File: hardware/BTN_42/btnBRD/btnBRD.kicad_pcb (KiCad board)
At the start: 2 copper layers, 113 parts, among them J1 Jack-DC, J10 Display Jumper, J2 MIDI-IN, J3 MIDI-OUT, J4 AudioJack2, J5 AudioJack2, J6 AudioJack2, J7 AudioJack2, J8 AudioJack2, J9 AudioJack2, SW1 SW_Push, SW10 SW_Push, SW11 SW_Push, SW12 SW_Push, SW13 SW_Push, SW14 SW_Push, SW15 SW_Push, SW16 SW_Push, SW17 SW_Push, SW18 SW_Push, SW19 SW_Push, SW2 SW_Push, SW20 SW_Push, SW21 SW_Push, SW22 SW_Push, SW23 SW_Push, SW24 SW_Push, SW25 SW_Push, SW26 SW_Push, SW27 SW_Push, SW28 SW_Push, SW29 SW_Push, SW3 SW_Push, SW30 SW_Push, SW31 SW_Push, SW32 SW_Push, SW33 SW_Push, SW34 SW_Push, SW35 SW_Push, SW36 SW_Push, SW37 SW_Push, SW38 SW_Push, SW39 SW_Push, SW4 SW_Push, SW40 SW_Push, SW41 SW_Push, SW42 SW_Push, SW43 SW_Push, SW44 SW_Push, SW45 SW_Push, SW46 SW_Push, SW47 SW_Push, SW48 SW_Push, SW5 SW_Push, SW6 SW_Push, SW7 SW_Push, SW8 SW_Push, SW9 SW_Push, U1 brain, U2 CD74HC4067M, U3 CD74HC4067M, U4 TXB0108DQSR

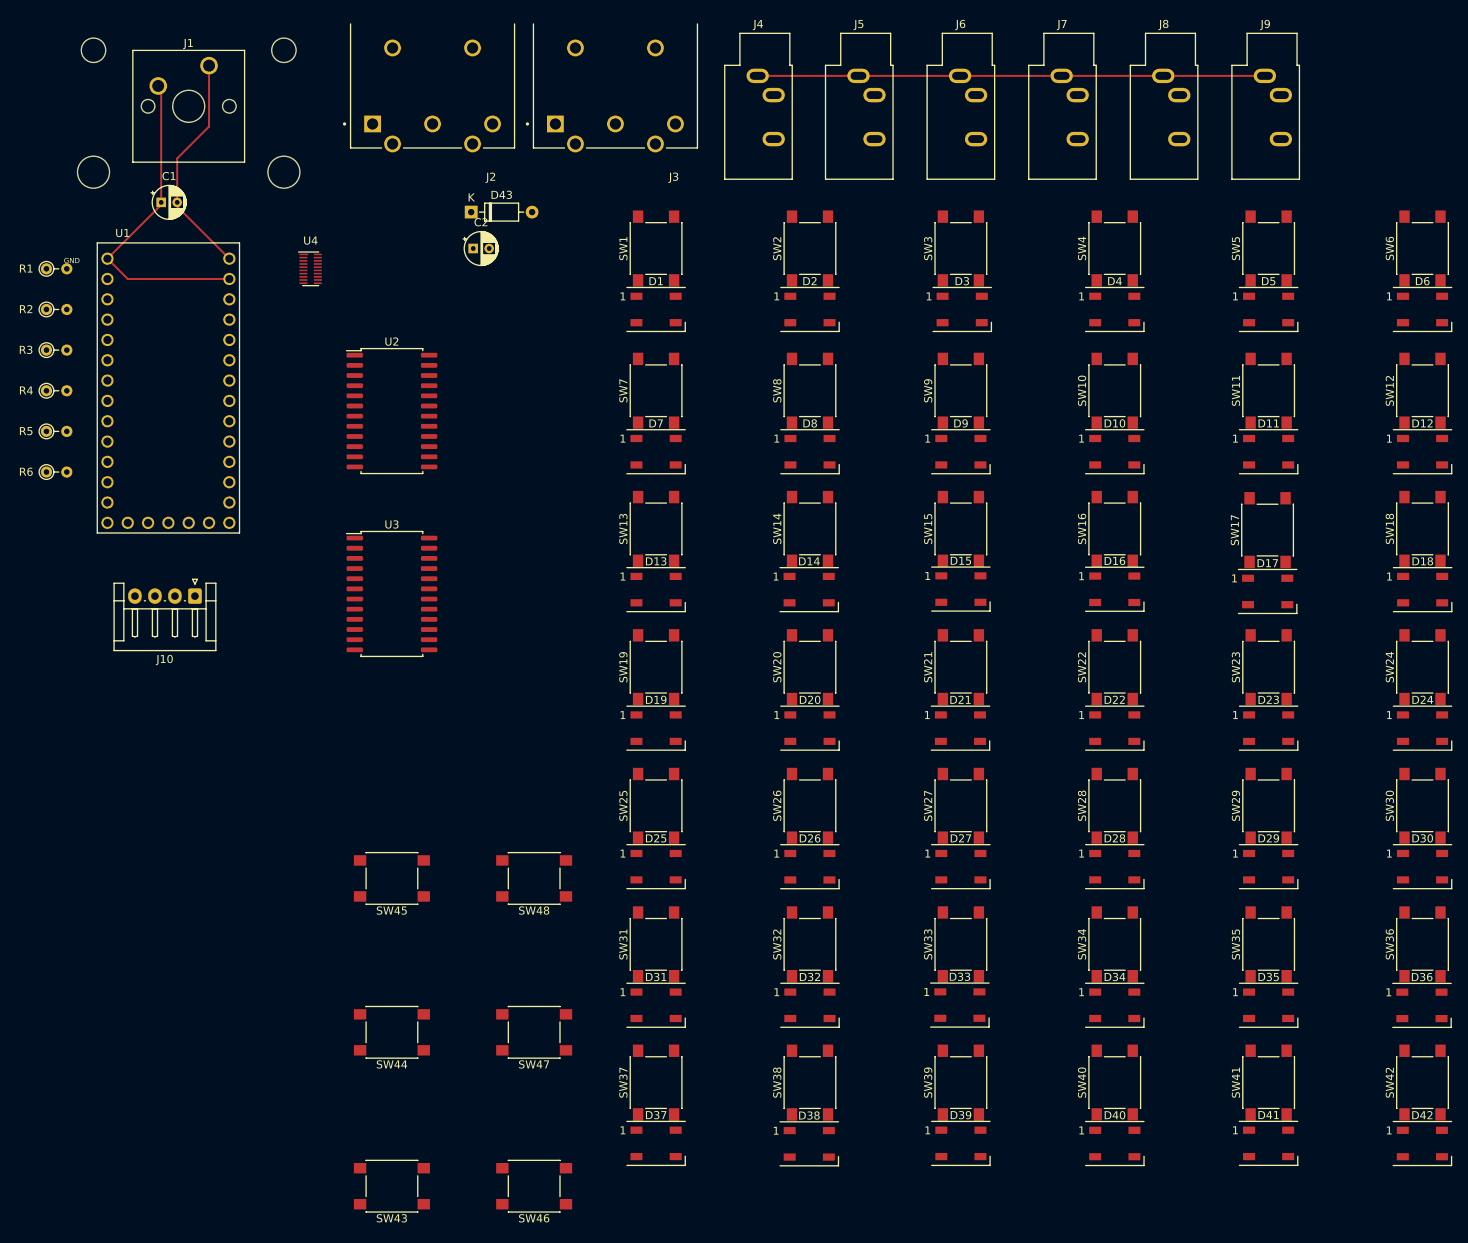
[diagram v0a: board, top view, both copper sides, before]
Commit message: brddd
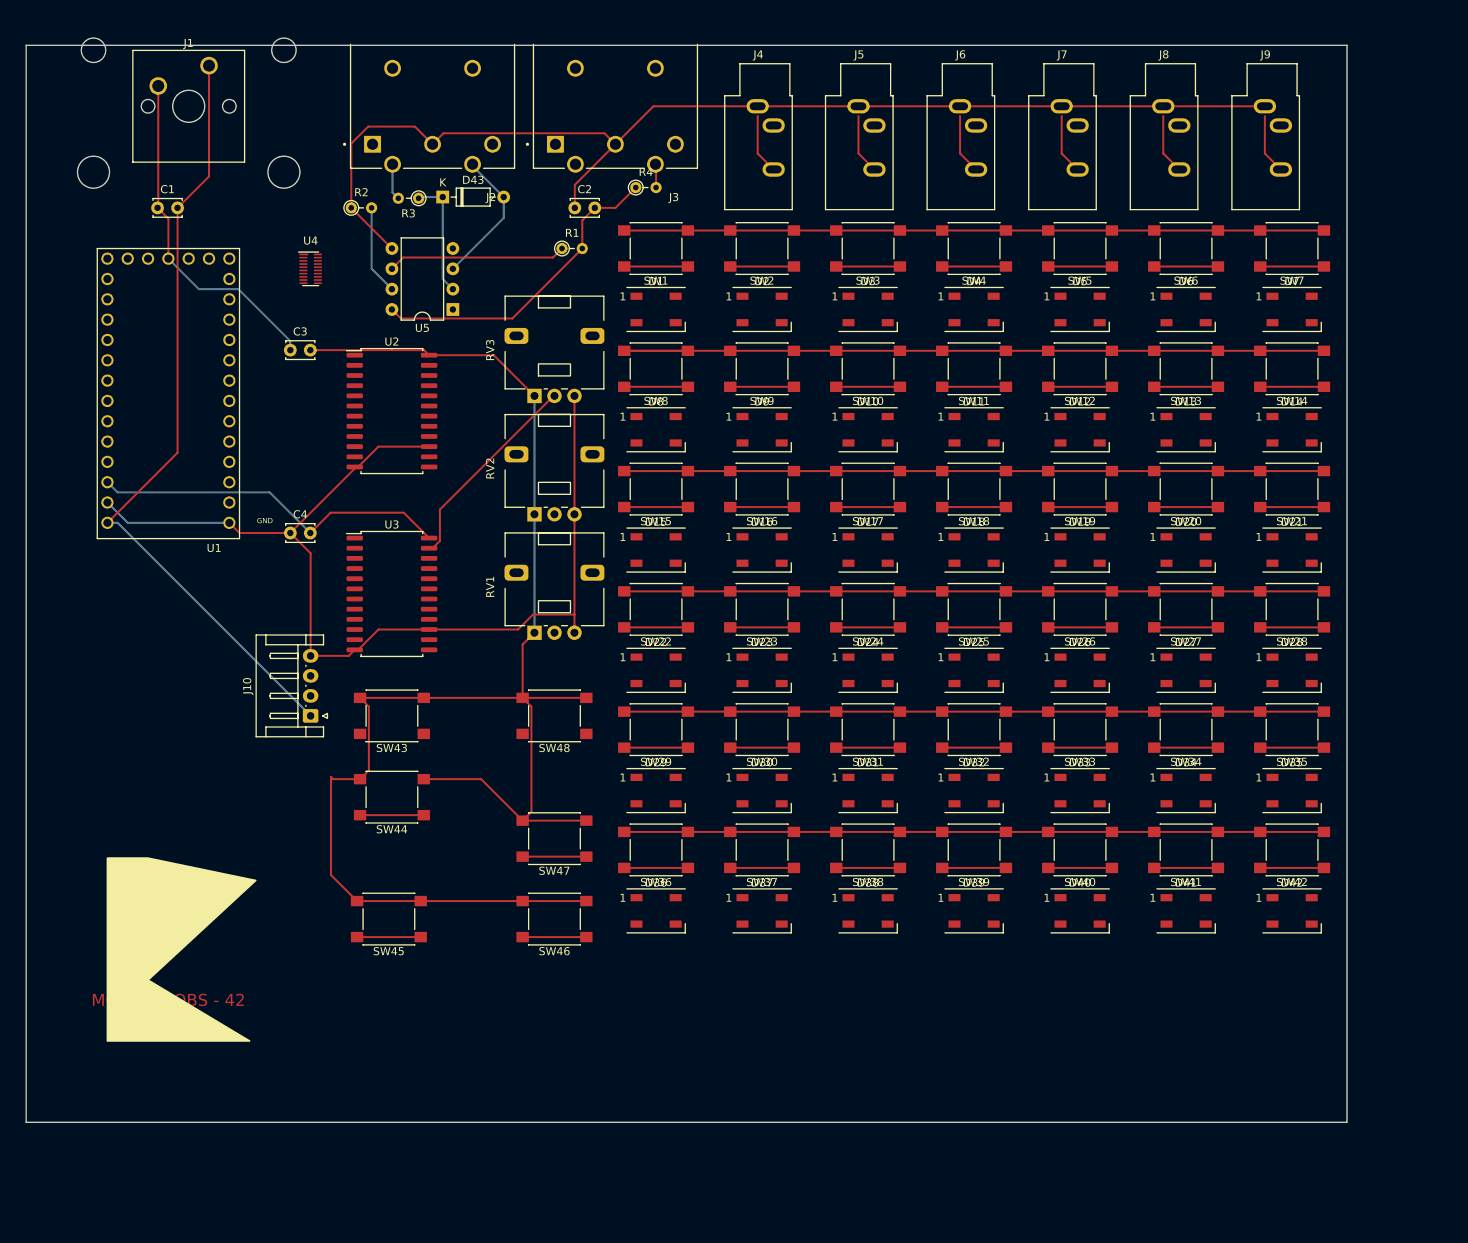
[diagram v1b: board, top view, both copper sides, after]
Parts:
- removed R5, R6: 10k, Resistor_THT:R_Axial_DIN0204_L3.6mm_D1.6mm_P2.54mm_Vertical
- added C3: 100nF, Capacitor_THT:C_Disc_D3.4mm_W2.1mm_P2.50mm, F.Cu at (48.3, 55.9)
- added C4: 100nF, Capacitor_THT:C_Disc_D3.4mm_W2.1mm_P2.50mm, F.Cu at (48.3, 78.7)
- added RV1: 10k - ff, Potentiometer_THT:Potentiometer_Alps_RK09L_Single_Vertical, F.Cu at (78.8, 91.2)
- added RV2: 10k - q, Potentiometer_THT:Potentiometer_Alps_RK09L_Single_Vertical, F.Cu at (78.8, 76.4)
- added RV3: 10k - main, Potentiometer_THT:Potentiometer_Alps_RK09L_Single_Vertical, F.Cu at (78.8, 61.6)
- added U5: 6N138, Package_DIP:DIP-8_W7.62mm, F.Cu at (68.6, 50.8)
- C1: footprint Capacitor_THT:CP_Radial_D4.0mm_P2.00mm -> Capacitor_THT:C_Disc_D3.4mm_W2.1mm_P2.50mm
- C2: value 10uF -> 470uF; footprint Capacitor_THT:CP_Radial_D4.0mm_P2.00mm -> Capacitor_THT:C_Disc_D3.4mm_W2.1mm_P2.50mm
- R1, R3, R4: value 10k -> 220
- R2: value 10k -> 4.7k
- SW1: value SW_Push -> 1x1
- SW10: value SW_Push -> 3x2
- SW11: value SW_Push -> 4x2
- SW12: value SW_Push -> 5x2
- SW13: value SW_Push -> 6x2
- SW14: value SW_Push -> 7x2
- SW15: value SW_Push -> 1x3
- SW16: value SW_Push -> 2x3
- SW17: value SW_Push -> 3x3
- SW18: value SW_Push -> 4x3
- SW19: value SW_Push -> 5x3
- SW2: value SW_Push -> 2x1
- SW20: value SW_Push -> 6x3
- SW21: value SW_Push -> 7x3
- SW22: value SW_Push -> 1x4
- SW23: value SW_Push -> 2x4
- SW24: value SW_Push -> 3x4
- SW25: value SW_Push -> 4x4
- SW26: value SW_Push -> 5x4
- SW27: value SW_Push -> 6x4
- SW28: value SW_Push -> 7x4
- SW29: value SW_Push -> 1x5
- SW3: value SW_Push -> 3x1
- SW30: value SW_Push -> 2x5
- SW31: value SW_Push -> 3x5
- SW32: value SW_Push -> 4x5
- SW33: value SW_Push -> 5x5
- SW34: value SW_Push -> 6x5
- SW35: value SW_Push -> 7x5
- SW36: value SW_Push -> 1x6
- SW37: value SW_Push -> 2x6
- SW38: value SW_Push -> 3x6
- SW39: value SW_Push -> 4x6
- SW4: value SW_Push -> 4x1
- SW40: value SW_Push -> 5x6
- SW41: value SW_Push -> 6x6
- SW42: value SW_Push -> 7x6
- SW43: value SW_Push -> cntrl1
- SW44: value SW_Push -> cntrl2
- SW45: value SW_Push -> cntrl3
- SW46: value SW_Push -> cntrl4
- SW47: value SW_Push -> cntrl5
- SW48: value SW_Push -> cntrl6
- SW5: value SW_Push -> 5x1
- SW6: value SW_Push -> 6x1
- SW7: value SW_Push -> 7x1
- SW8: value SW_Push -> 1x2
- SW9: value SW_Push -> 2x2
- U1: value brain -> brain - teensy 4.0
- U2: value CD74HC4067M -> digital mux - 74hc4067m
- U3: value CD74HC4067M -> analog mux - 74hc4067m
- moved SW36 96.5 mm to (94.0, 118.4), turned to 180 degrees
- moved D36 96.5 mm to (94.0, 126.0)
- moved SW30 83.1 mm to (107.2, 103.3), turned to 180 degrees
- moved D30 83.1 mm to (107.2, 110.9)
- moved D7 81.5 mm to (173.5, 50.8)
- moved SW7 81.5 mm to (173.5, 43.2), turned to 180 degrees
- moved R4 77.9 mm to (91.4, 35.6)
- moved SW29 77.2 mm to (94.0, 103.3), turned to 180 degrees
- moved D29 77.2 mm to (94.0, 110.9)
- moved D24 69.7 mm to (120.5, 95.9)
- moved SW24 69.7 mm to (120.5, 88.3), turned to 180 degrees
- moved SW13 69.2 mm to (160.2, 58.2), turned to 180 degrees
- moved D13 69.2 mm to (160.2, 65.8)
- moved R1 64.5 mm to (82.2, 43.2)
- moved D23 63.7 mm to (107.2, 95.9)
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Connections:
- R1 pad 1: Ctrl1 -> MIDI_IN
- R1 pad 2: 3VDC -> 5VDC
- R2 pad 1: Ctrl2 -> GND
- R2 pad 2: 3VDC -> Net-(R2-Pad2)
- R3 pad 1: Ctrl3 -> Net-(D43-Pad1)
- R3 pad 2: 3VDC -> Net-(J2-Pad4)
- R4 pad 1: Ctrl4 -> 5VDC
- R4 pad 2: 3VDC -> Net-(J3-Pad5)
- SW1 pad 2: 3VDC -> col1
- SW10 pad 2: 3VDC -> col2
- SW11 pad 2: 3VDC -> col2
- SW12 pad 2: 3VDC -> col2
- SW13 pad 2: 3VDC -> col2
- SW14 pad 2: 3VDC -> col2
- SW15 pad 2: 3VDC -> col3
- SW16 pad 2: 3VDC -> col3
- SW17 pad 2: 3VDC -> col3
- SW18 pad 2: 3VDC -> col3
- SW19 pad 2: 3VDC -> col3
- SW2 pad 2: 3VDC -> col1
- SW20 pad 2: 3VDC -> col3
- SW21 pad 2: 3VDC -> col3
- SW22 pad 2: 3VDC -> col4
- SW23 pad 2: 3VDC -> col4
- SW24 pad 2: 3VDC -> col4
- SW25 pad 2: 3VDC -> col4
- SW26 pad 2: 3VDC -> col4
- SW27 pad 2: 3VDC -> col4
- SW28 pad 2: 3VDC -> col4
- SW29 pad 2: 3VDC -> col5
- SW3 pad 2: 3VDC -> col1
- SW30 pad 2: 3VDC -> col5
- SW31 pad 2: 3VDC -> col5
- SW32 pad 2: 3VDC -> col5
- SW33 pad 2: 3VDC -> col5
- SW34 pad 2: 3VDC -> col5
- SW35 pad 2: 3VDC -> col5
- SW36 pad 2: 3VDC -> col6
- SW37 pad 2: 3VDC -> col6
- SW38 pad 2: 3VDC -> col6
- SW39 pad 2: 3VDC -> col6
- SW4 pad 2: 3VDC -> col1
- SW40 pad 2: 3VDC -> col6
- SW41 pad 2: 3VDC -> col6
- SW42 pad 2: 3VDC -> col6
- SW5 pad 2: 3VDC -> col1
- SW6 pad 2: 3VDC -> col1
- SW7 pad 2: 3VDC -> col1
- SW8 pad 2: 3VDC -> col2
- SW9 pad 2: 3VDC -> col2
- U1 pad 10: MuxC1 -> MuxC3
- U1 pad 11: MuxC2 -> MuxC4
- U1 pad 12: MuxC3 -> unconnected-(U1-Pad12)
- U1 pad 2: unconnected-(U1-Pad2) -> MuxR1
- U1 pad 3: unconnected-(U1-Pad3) -> MuxR2
- U1 pad 4: unconnected-(U1-Pad4) -> MuxR3
- U1 pad 5: unconnected-(U1-Pad5) -> MuxR4
- U1 pad 7: MuxR1 -> unconnected-(U1-Pad7)
- U1 pad 8: MuxR2 -> MuxC1
- U1 pad 9: MuxR3 -> MuxC2
- U2 pad 1: GND -> MRR
- U2 pad 10: MRR -> MuxR1
- U2 pad 11: MuxR1 -> MuxR2
- U2 pad 13: MuxR3 -> MuxR4
- U2 pad 14: MuxR2 -> MuxR3
- U2 pad 19: unconnected-(U2-Pad19) -> col6
- U2 pad 2: Ctrl3 -> col1
- U2 pad 20: unconnected-(U2-Pad20) -> col5
- U2 pad 21: unconnected-(U2-Pad21) -> col4
- U2 pad 22: Ctrl1 -> col3
- U2 pad 23: Ctrl2 -> col2
- U3 pad 1: GND -> MRC
- U3 pad 10: MRC -> MuxC1
- U3 pad 11: MuxC1 -> MuxC2
- U3 pad 13: MuxC3 -> MuxC4
- U3 pad 14: MuxC2 -> MuxC3
- U3 pad 2: Ctrl5 -> fp2
- U3 pad 23: Ctrl4 -> main
- U3 pad 4: col6 -> Ctrl5
- U3 pad 5: col5 -> Ctrl4
- U3 pad 6: col4 -> Ctrl3
- U3 pad 7: col3 -> Ctrl2
- U3 pad 8: col2 -> Ctrl1
- U3 pad 9: col1 -> fp1
- U4 pad 6: unconnected-(U4-Pad6) -> GND
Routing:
- net 3VDC: track 0.00 -> 241.5 mm
- net GND: track 104.2 -> 315.2 mm
- net 5VDC: track 28.5 -> 137.6 mm
- net col2: track 0.00 -> 95.4 mm
- net col6: track 0.00 -> 87.5 mm
- net col5: track 0.00 -> 87.5 mm
- net col4: track 0.00 -> 87.5 mm
- net col3: track 0.00 -> 87.5 mm
- net col1: track 0.00 -> 87.0 mm
- net row2: track 0.00 -> 48.5 mm
- net row7: track 0.00 -> 47.8 mm
- net row6: track 0.00 -> 47.8 mm
- net row5: track 0.00 -> 47.8 mm
- net row4: track 0.00 -> 47.8 mm
- net row3: track 0.00 -> 47.8 mm
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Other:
- board outline added: 165.1 x 134.6 mm
- board text added: "MOAR k NOBS - 42"
